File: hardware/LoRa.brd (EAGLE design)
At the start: 47 x 40.5 mm, 26 parts, among them J1 U.FL-R-SMT, J2 U.FL-R-SMT, J3 U.FL-R-SMT, U1 E220-900T22S, U2 E220-900T22S

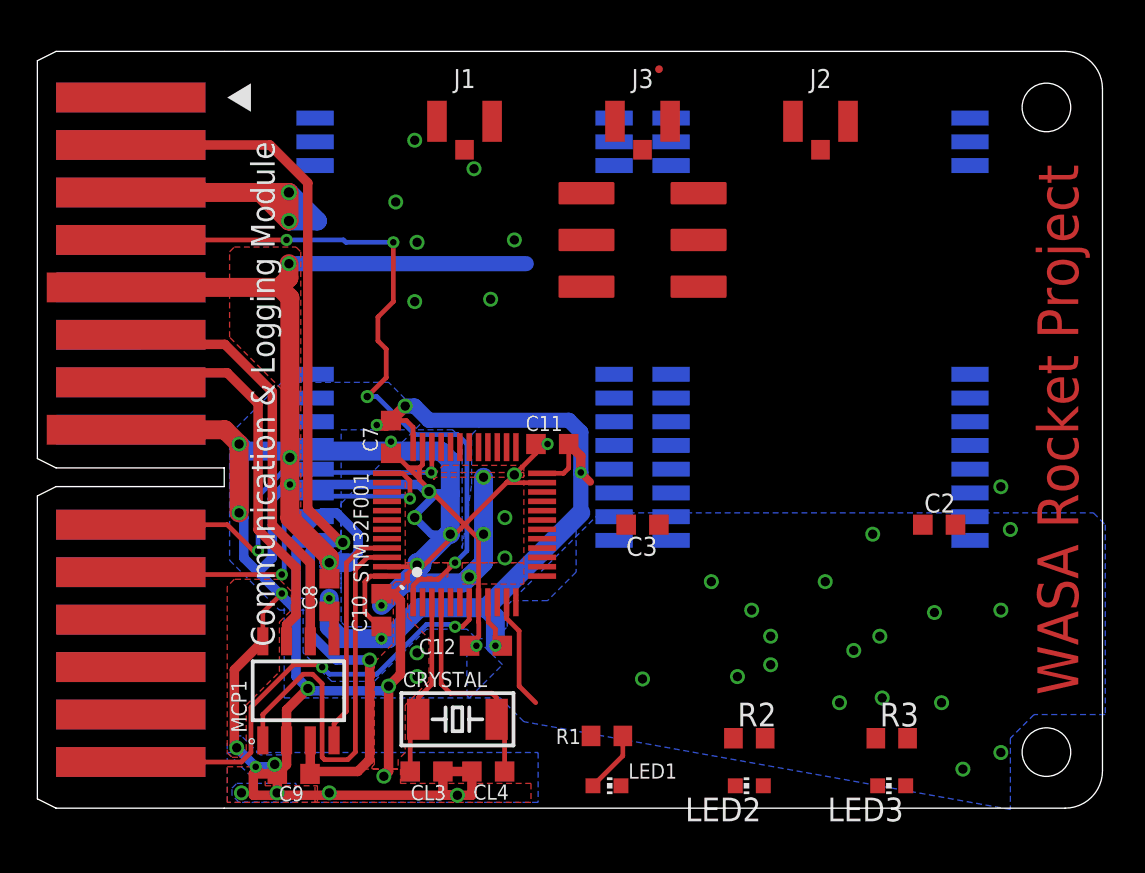
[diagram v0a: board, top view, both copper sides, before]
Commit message: LoRaモジュール、基板設計完了です。
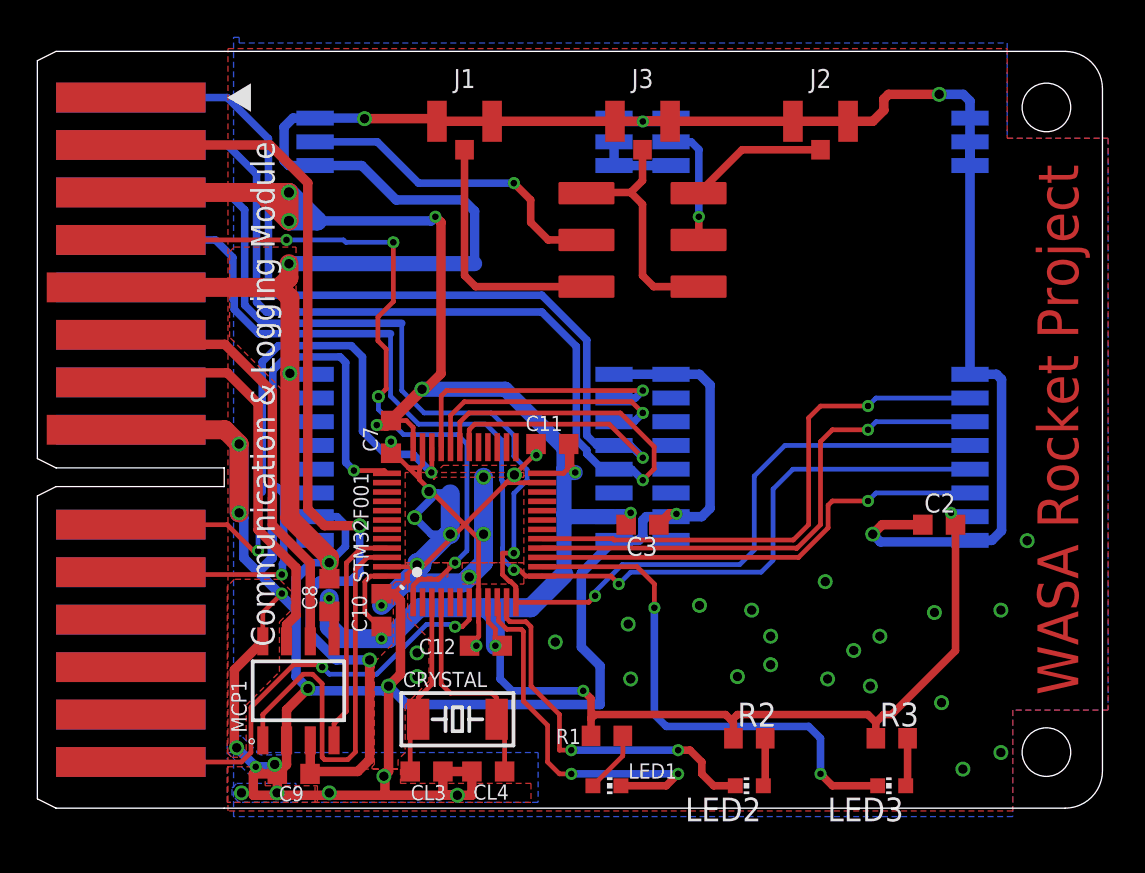
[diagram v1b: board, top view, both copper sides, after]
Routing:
- net GND: track 208.5 -> 325.5 mm, vias 59 -> 54
- net LORA2_TRX: track 0.00 -> 71.7 mm, vias 0 -> 2
- net LORA2_RTX: track 0.00 -> 64.8 mm, vias 0 -> 2
- net VDD: track 71.9 -> 135.5 mm, vias 8 -> 12
- net LORA1_RTX: track 0.00 -> 56.6 mm, vias 0 -> 1
- net LORA1_TRX: track 0.00 -> 54.4 mm, vias 0 -> 1
- net LORA2_M0: track 0.00 -> 29.4 mm, vias 0 -> 1
- net LORA2_M1: track 0.00 -> 28.3 mm, vias 0 -> 1
- net N$6: track 0.00 -> 28.0 mm, vias 0 -> 2
- net LORA2_AUX: track 0.00 -> 25.0 mm, vias 0 -> 1
- net N$10: track 0.00 -> 20.7 mm, vias 0 -> 2
- net N$1: track 0.00 -> 17.4 mm, vias 0 -> 1
- net LORA1_M0: track 0.00 -> 15.4 mm, vias 0 -> 1
- net LORA1_M1: track 0.00 -> 14.3 mm, vias 0 -> 1
- net N$73: track 6.02 -> 20.2 mm, vias 0 -> 2
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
